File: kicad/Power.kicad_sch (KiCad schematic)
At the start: 18 parts, among them J10 10137064-00021LF, J8 Conn_01x06_Pin, Q4 Si2319CDS, Q5 Si2319CDS, U2 CYPD3177-24LQ

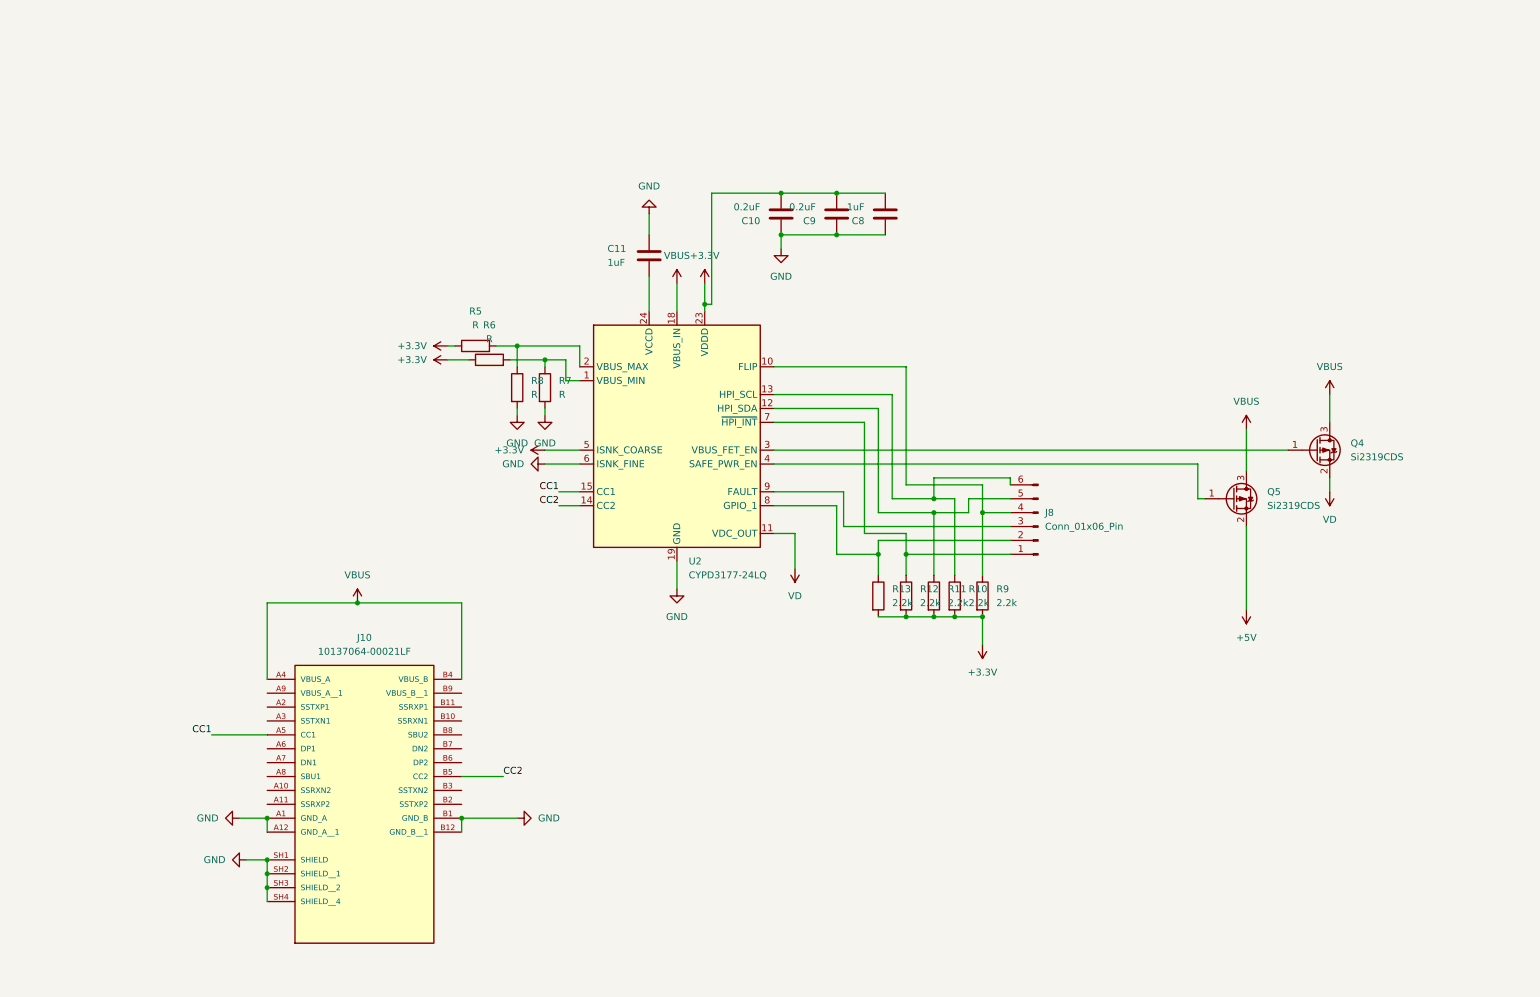
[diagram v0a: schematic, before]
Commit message: feat: v2
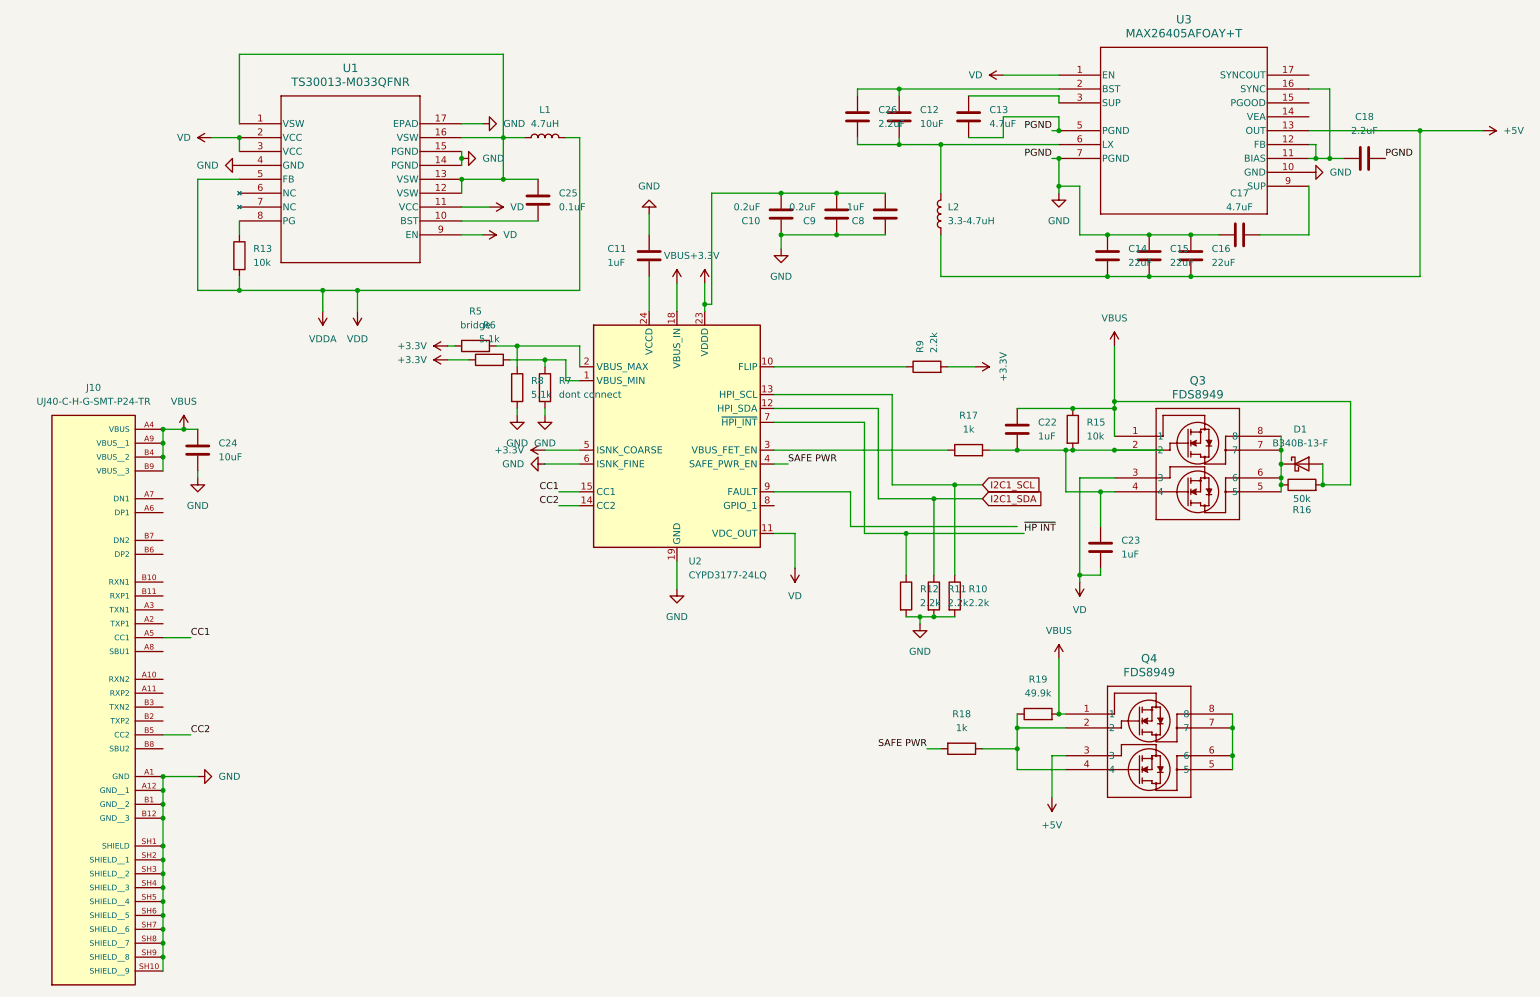
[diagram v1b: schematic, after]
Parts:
- removed J10: 10137064-00021LF, Ampheon-10137064-00021LF:AMPHENOL_10137064-00021LF, symbol 10137064-00021LF:10137064-00021LF
- removed J8: Conn_01x06_Pin, Connector_PinHeader_2.54mm:PinHeader_1x06_P2.54mm_Vertical, symbol Connector:Conn_01x06_Pin
- removed Q4: Si2319CDS, Package_TO_SOT_SMD:SOT-23-3, symbol Transistor_FET:Si2343CDS
- removed Q5: Si2319CDS, Package_TO_SOT_SMD:SOT-23, symbol Transistor_FET:Si2329CDS
- added C12: 10uF, Capacitor_SMD:C_0603_1608Metric, symbol Device:C
- added C13, C17: 4.7uF, Capacitor_SMD:C_0603_1608Metric, symbol Device:C
- added C14, C15, C16: 22uF, Capacitor_SMD:C_0805_2012Metric, symbol Device:C
- added C18, C26: 2.2uF, Capacitor_SMD:C_0603_1608Metric, symbol Device:C
- added C22, C23: 1uF, Capacitor_SMD:C_0805_2012Metric, symbol Device:C
- added C24: 10uF, Capacitor_SMD:C_0805_2012Metric, symbol Device:C
- added C25: 0.1uF, Resistor_SMD:R_0402_1005Metric, symbol Device:C
- added D1: B340B-13-F, Diode_SMD:D_SMB, symbol Device:D_Schottky
- added J10: UJ40-C-H-G-SMT-P24-TR, Own:SAMESKY_UJ40-C-H-G-SMT-P24-TR, symbol UJ40-C-H-G-SMT-P24-TR:UJ40-C-H-G-SMT-P24-TR
- added L1: 4.7uH, Own:IND_NRS5030T100MMGJ_TAY, symbol Device:L
- added L2: 3.3-4.7uH, Inductor_SMD:L_Coilcraft_XxL4030, symbol Device:L
- added Q3, Q4: FDS8949, Own:SOIC8_3P9X4P9_OSI, symbol FDS8949:FDS8949
- added R15: 10k, Capacitor_SMD:C_0603_1608Metric, symbol Device:R
- added R16: 50k, Resistor_SMD:R_0603_1608Metric, symbol Device:R
- added R17: 1k, Capacitor_SMD:C_0603_1608Metric, symbol Device:R
- added R18: 1k, Resistor_SMD:R_0402_1005Metric, symbol Device:R
- added R19: 49.9k, Resistor_SMD:R_0402_1005Metric, symbol Device:R
- added U1: TS30013-M033QFNR, Own:QFN16_3X3_SEM, symbol TS30011-M033QFNR:TS30013-M033QFNR
- added U3: MAX26405AFOAY+T, Own:FC2QFN-17, symbol Own:MAX26405AFOAY+T
- C10, C11, C8: footprint Capacitor_SMD:C_0603_1608Metric -> Capacitor_SMD:C_0402_1005Metric
- C9: footprint Resistor_SMD:R_0603_1608Metric -> Capacitor_SMD:C_0402_1005Metric
- R10, R11, R12, R9: footprint Resistor_SMD:R_0603_1608Metric -> Resistor_SMD:R_0402_1005Metric
- R13: value 2.2k -> 10k; footprint Resistor_SMD:R_0603_1608Metric -> Resistor_SMD:R_0402_1005Metric
- R5: value R -> bridge; footprint Resistor_SMD:R_0603_1608Metric -> Resistor_SMD:R_0402_1005Metric
- R6, R8: value R -> 5.1k; footprint Resistor_SMD:R_0603_1608Metric -> Resistor_SMD:R_0402_1005Metric
- R7: value R -> dont connect; footprint Resistor_SMD:R_0603_1608Metric -> Resistor_SMD:R_0402_1005Metric
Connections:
- net +3.3V: no longer R10.2, R11.2, R12.2, R13.2
- net +5V: now also C14.2, C15.2, C16.2, L2.1, Q4.3, U3.13 (OUT)
- net CC1: now also J10.A5 (CC1)
- net CC2: now also J10.B5 (CC2)
- net GND: now also R10.2, R11.2, R12.2, C13.2, C14.1, C15.1, C16.1, C17.1, C18.2, C24.1, J10.A1 (GND), J10.A12 (GND__1), J10.B1 (GND__2), J10.B12 (GND__3), J10.SH1 (SHIELD), J10.SH10 (SHIELD__9), J10.SH2 (SHIELD__1), J10.SH3 (SHIELD__2), J10.SH4 (SHIELD__3), J10.SH5 (SHIELD__4), J10.SH6 (SHIELD__5), J10.SH7 (SHIELD__6), J10.SH8 (SHIELD__7), J10.SH9 (SHIELD__8), U1.14 (PGND), U1.15 (PGND), U1.17 (EPAD), U1.4 (GND), U3.10 (GND), U3.5 (PGND), U3.7 (PGND)
- net VBUS: now also C22.1, C24.2, D1.2 (A), J10.A4 (VBUS), J10.A9 (VBUS__1), J10.B4 (VBUS__2), J10.B9 (VBUS__3), Q3.1, Q4.1, R15.1, R16.2, R19.2
- net VD: now also C23.2, Q3.3, U1.11 (VCC), U1.2 (VCC), U1.3 (VCC), U1.9 (EN), U3.1 (EN)
- net I2C1_SCL: now reaches R10.1, U2.13 (HPI_SCL)
- net ~{HP INT}: now reaches R12.1, U2.7 (~{HPI_INT})
- net at R13.1: now also U1.8 (PG); no longer U2.8 (GPIO_1)
- net I2C1_SDA: now reaches R11.1, U2.12 (HPI_SDA)
- net SAFE PWR: now reaches U2.4 (SAFE_PWR_EN)
- net SAFE PWR: now also R18.2
- net at U2.3 (VBUS_FET_EN): now also R17.1
- new net: C25.1, L1.1, U1.1 (VSW), U1.12 (VSW), U1.13 (VSW), U1.16 (VSW)
- new net: C25.2, U1.10 (BST)
- new net: C22.2, C23.1, Q3.2, Q3.4, R15.2, R17.2
- new net: D1.1 (K), Q3.5, Q3.6, Q3.7, Q3.8, R16.1
- new net: C12.1, C26.1, U3.2 (BST)
- new net: C12.2, C26.2, L2.2, U3.6 (LX)
- new net: C17.2, U3.9 (SUP)
- new net: Q4.2, Q4.4, R18.1, R19.1
- new net: Q4.5, Q4.6, Q4.7, Q4.8
- new net: C18.1, U3.11 (BIAS), U3.12 (FB), U3.16 (SYNC)
- new net: C13.1, U3.3 (SUP)
- new net VDD: L1.2, R13.2, U1.5 (FB)
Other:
- moved on the sheet: R9
